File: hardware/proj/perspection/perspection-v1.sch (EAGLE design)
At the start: 232 parts, among them J1 MICRO-USB-10118192-0001LF, J2 1X6-PTSA_1.5/6-3.5-Z, J3 1X2-PTSA_1.5/2-3.5-Z, J4 1X2-JST-PH-SMD, J5 1X2-0428202213, J6 JTAG-ARM_TC-10, J7 JTAG-ARM_TC-10, Q1 NMOS-CSD18533Q5A, Q10 NMOS-CSD18533Q5A, Q11 IRFML8244TRPBF, Q2 NMOS-CSD18533Q5A, Q3 NMOS-CSD18533Q5A, Q4 NMOS-CSD18533Q5A, Q5 NMOS-CSD18533Q5A, Q6 NMOS-CSD18533Q5A, Q7 NMOS-CSD18533Q5A, Q8 BSS138L, Q9 BSS138L, U1 ATUM, U10 DRV8301DCAR, U11 OPA2374AIDCNR, U12 OPA170AIDBVR, U13 BNO055, U2 FT232RQ, U3 TPS79933DDCR, U4 MCP73831T-2ACI/OT, U5 TMS320F28069MPZT, U6 DRV8801PWPR, U7 DRV8801PWPR, U8 DRV8801PWPR, U9 DRV8801PWPR, Y1 32.768kHz

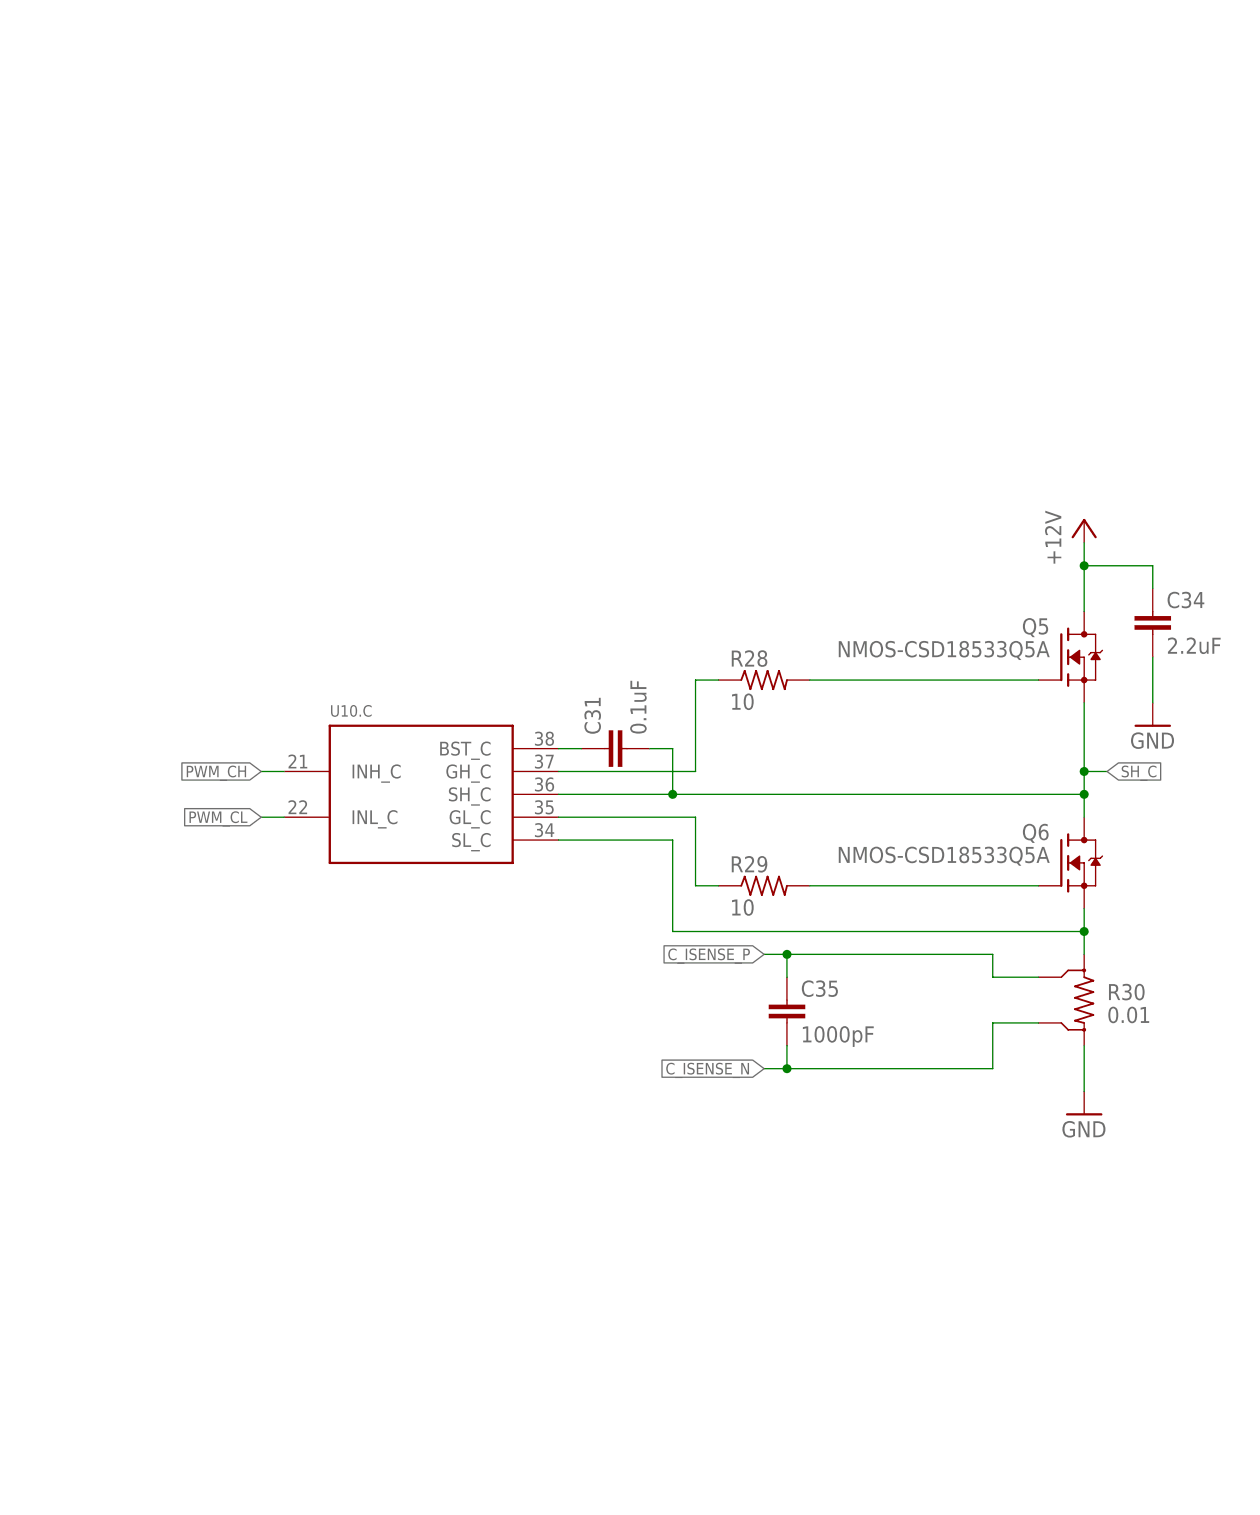
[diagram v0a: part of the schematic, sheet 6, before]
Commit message: boz is making me commit
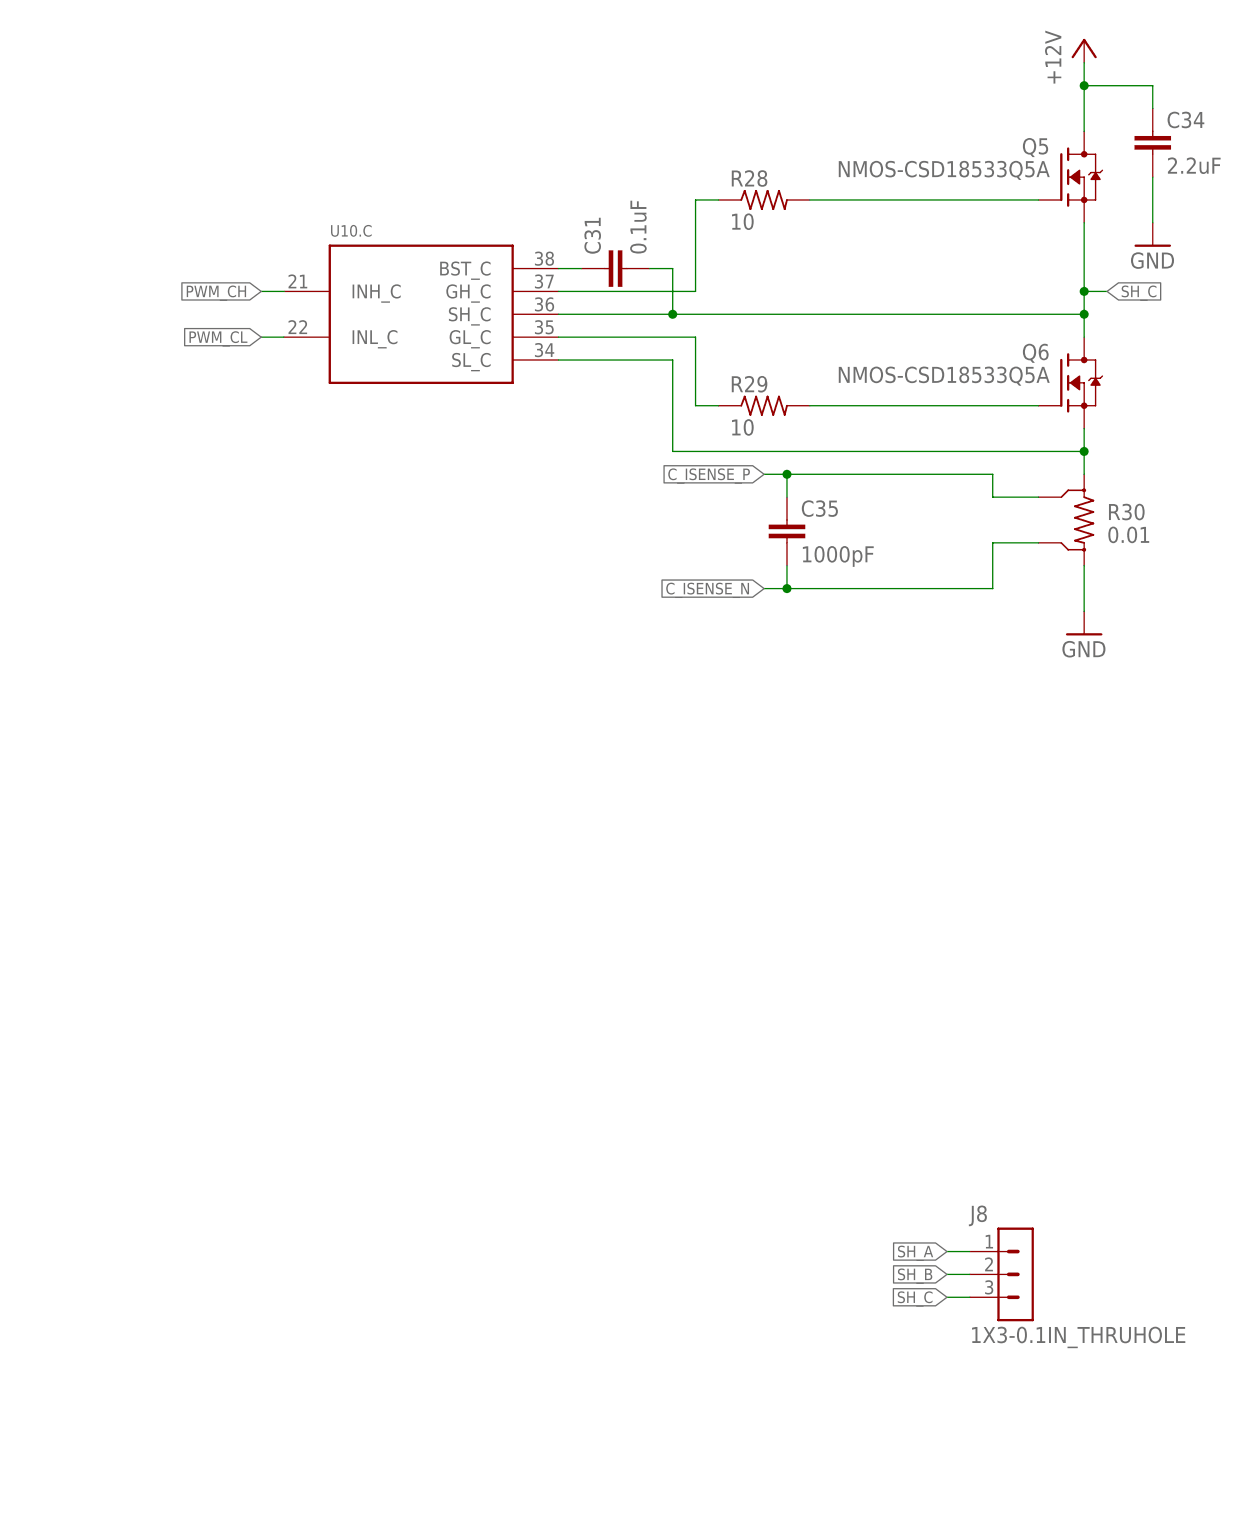
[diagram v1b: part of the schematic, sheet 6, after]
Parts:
- added J8: 1X3-0.1IN_THRUHOLE, perspection:1X3-0.1IN_THRUHOLE
- C20, C21, C22, C26, C37, C38, C6: device perspection:C0603 -> perspection:C0402
- C45, C57: device perspection:C0805 -> perspection:C0402
- R22, R27, R30: device perspection:R-SENSE3637-0.01 -> perspection:R-SENSE2010-0.01
- R83, R84, R85, R86, R87, R88: device perspection:R0603 -> perspection:R0402
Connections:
- net N$43 renamed DVDD
- net N$44 renamed AVDD
- net N$46 renamed PH
- net N$47 renamed RT_CLK
- net N$48 renamed BST_BK
- net N$49 renamed DTC
- net N$50 renamed SS_TR
- net N$52 renamed PWRGD
- net N$53 renamed GVDD
- net N$54 renamed _COMP
- net N$55 renamed COMP
- net N$57 renamed VFB
- net N$86 renamed +12V_GND
- net N$88 renamed VBAT_GND
- net GND: now also D6.HEAT
- net SH_A: now also J8.1
- net SH_B: now also J8.2
- net SH_C: now also J8.3
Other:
- moved on the sheet: C31, C34, C35, D6, Q5, Q6, R28, R29, R30, U10.C
